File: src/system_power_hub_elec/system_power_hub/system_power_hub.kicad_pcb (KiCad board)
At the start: 6 copper layers, 65 x 65 mm, 127 parts, among them J1 XT90M, J101 SM02B-PASS, J2 XT60F, J3 SM02B-PASS, J4 XT60F, J6 IDC6, J8 XT60F, J9 XT60F, Q1 SSM3K333R, Q10 IRFH7440TRPBF, Q2 Q_Dual_NPN_NPN_E1B1C2E2B2C1, Q3 IRFH7440TRPBF, Q4 IRFH7440TRPBF, Q8 Q_Dual_NPN_NPN_E1B1C2E2B2C1, Q9 IRFH7440TRPBF, U102 TCAN1462V, U2 STM32G474RBT6, U220 MP2459GJ-Z-MS, U230 AP62200TWU, U4 24LC128, Y1 24MHz

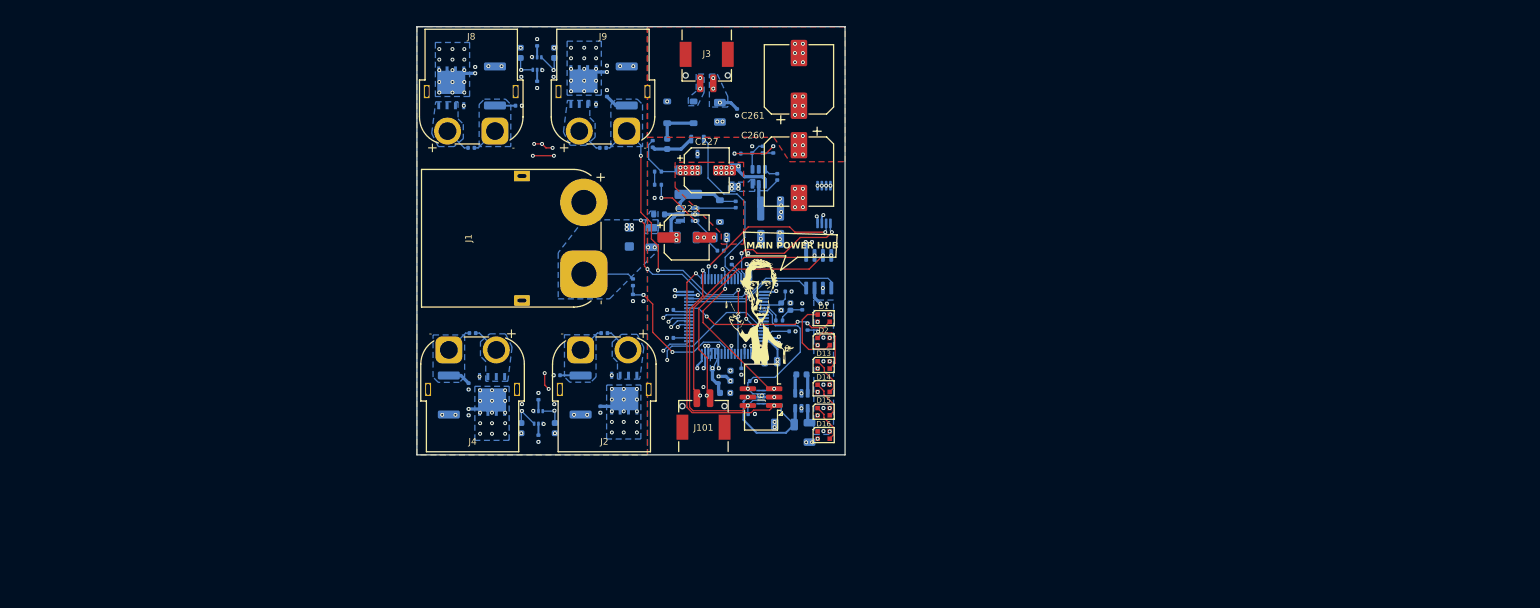
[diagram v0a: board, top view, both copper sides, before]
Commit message: Draft SPM PCB layout
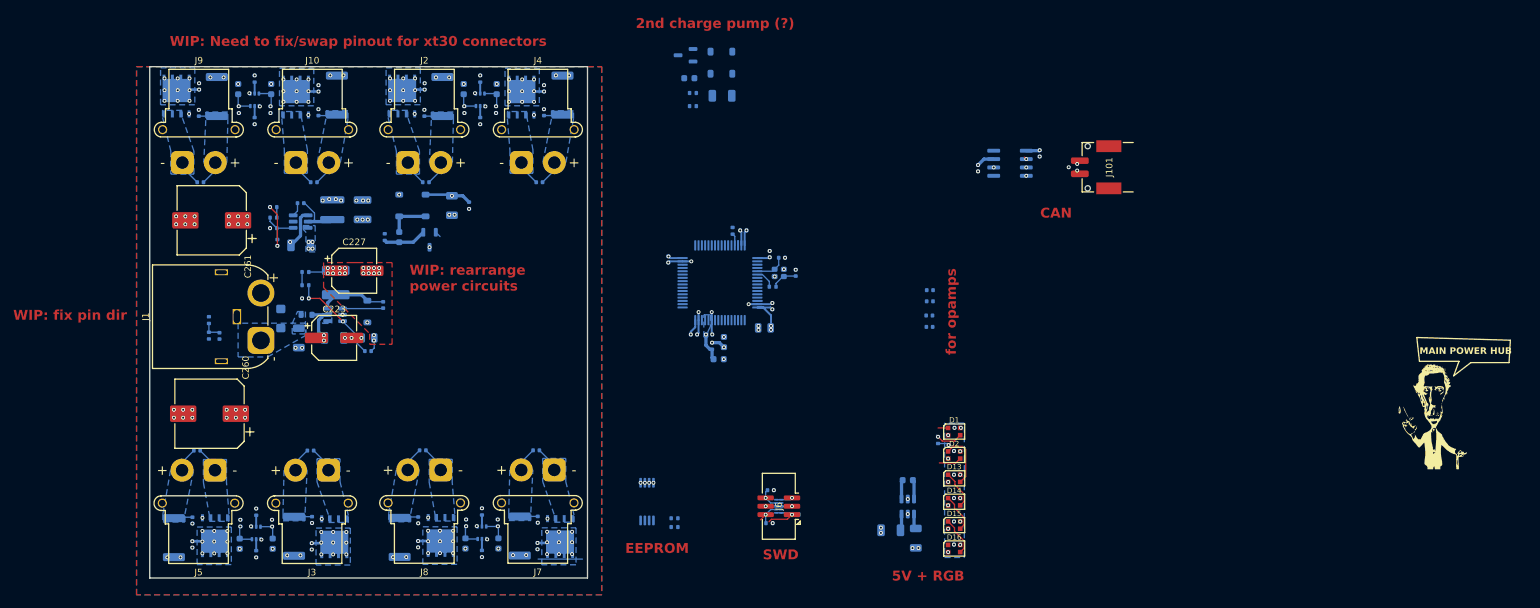
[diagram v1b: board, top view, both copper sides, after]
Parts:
- removed U2: STM32G474RBT6, Package_QFP:LQFP-64_10x10mm_P0.5mm
- added C32: 100n, Capacitor_SMD:C_0603_1608Metric, B.Cu at (141.4, 57.8)
- added C33: 1u, Capacitor_SMD:C_1206_3216Metric, B.Cu at (146.3, 60.5)
- added C34: 100n, Capacitor_SMD:C_0603_1608Metric, B.Cu at (78.1, 128.5)
- added C35: 100n, Capacitor_SMD:C_0603_1608Metric, B.Cu at (73.1, 128.5)
- added C38: 1n, Capacitor_SMD:C_0402_1005Metric, B.Cu at (83.8, 114.4)
- added C39: 1n, Capacitor_SMD:C_0402_1005Metric, B.Cu at (84.1, 124.9)
- added C40: 1n, Capacitor_SMD:C_0402_1005Metric, B.Cu at (66.6, 114.4)
- added C41: 1n, Capacitor_SMD:C_0402_1005Metric, B.Cu at (65.9, 125.0)
- added C42: 100n, Capacitor_SMD:C_0603_1608Metric, B.Cu at (112.4, 128.4)
- added C43: 100n, Capacitor_SMD:C_0603_1608Metric, B.Cu at (107.4, 128.5)
- added C44: 1n, Capacitor_SMD:C_0402_1005Metric, B.Cu at (118.1, 114.3)
- added C45: 1n, Capacitor_SMD:C_0402_1005Metric, B.Cu at (118.3, 124.8)
- added C46: 1n, Capacitor_SMD:C_0402_1005Metric, B.Cu at (100.9, 114.3)
- added C47: 1n, Capacitor_SMD:C_0402_1005Metric, B.Cu at (100.2, 124.9)
- added C48: 1n, Capacitor_SMD:C_0402_1005Metric, B.Cu at (118.3, 128.9)
- added C49: 1n, Capacitor_SMD:C_0402_1005Metric, B.Cu at (100.2, 128.6)
- added C50: 1n, Capacitor_SMD:C_0402_1005Metric, B.Cu at (84.0, 128.9)
- added C51: 1n, Capacitor_SMD:C_0402_1005Metric, B.Cu at (65.9, 128.6)
- added D4: SBR0560S1-7, Diode_SMD:D_SOD-123, B.Cu at (146.2, 53.8)
- added D5: SBR0560S1-7, Diode_SMD:D_SOD-123, B.Cu at (146.2, 57.1)
- added J5: XT30F, Connector_AMASS:AMASS_XT30PW-F_1x02_P2.50mm_Horizontal, F.Cu at (69.3, 117.3)
- added J7: XT30F, Connector_AMASS:AMASS_XT30PW-F_1x02_P2.50mm_Horizontal, F.Cu at (120.8, 117.3)
- added J8: XT30F, Connector_AMASS:AMASS_XT30PW-F_1x02_P2.50mm_Horizontal, F.Cu at (103.6, 117.3)
- added Q10: IRFH7440TRPBF, Bluesat:PQFN_5x6mm_E_SGD, B.Cu at (103.6, 127.6)
- added Q11: IRFH7440TRPBF, Bluesat:PQFN_5x6mm_E_SGD, B.Cu at (69.4, 127.6)
- added Q5: SSM3K333R, Package_TO_SOT_SMD:SOT-23-3, B.Cu at (140.8, 54.3)
- added Q6: Q_Dual_NPN_NPN_E1B1C2E2B2C1, Package_TO_SOT_SMD:SOT-363_SC-70-6, B.Cu at (75.6, 126.9)
- added Q7: IRFH7440TRPBF, Bluesat:PQFN_5x6mm_E_SGD, B.Cu at (87.5, 127.8)
- added Q8: Q_Dual_NPN_NPN_E1B1C2E2B2C1, Package_TO_SOT_SMD:SOT-363_SC-70-6, B.Cu at (109.9, 126.8)
- added Q9: IRFH7440TRPBF, Bluesat:PQFN_5x6mm_E_SGD, B.Cu at (121.7, 127.7)
- added R16: 10k, Resistor_SMD:R_0402_1005Metric, B.Cu at (109.9, 130.0)
- added R18: 100R, Resistor_SMD:R_0402_1005Metric, B.Cu at (141.9, 60.1)
- added R20: 470k, Resistor_SMD:R_0402_1005Metric, B.Cu at (141.9, 62.1)
- added R21: 10k, Resistor_SMD:R_0402_1005Metric, B.Cu at (109.9, 123.6)
- added R22: 470k, Resistor_SMD:R_0402_1005Metric, B.Cu at (112.3, 125.3)
- added R23: 470k, Resistor_SMD:R_0402_1005Metric, B.Cu at (107.5, 125.3)
- added R24: 10k, Resistor_SMD:R_0402_1005Metric, B.Cu at (75.6, 130.1)
- added R25: 10k, Resistor_SMD:R_0402_1005Metric, B.Cu at (75.6, 123.7)
- added R26: 1m, Resistor_SMD:R_2512_6332Metric, B.Cu at (115.6, 127.3)
- added R27: 1m, Resistor_SMD:R_2512_6332Metric, B.Cu at (97.4, 127.5)
- added R28: 470k, Resistor_SMD:R_0402_1005Metric, B.Cu at (78.0, 125.4)
- added R29: 470k, Resistor_SMD:R_0402_1005Metric, B.Cu at (73.2, 125.4)
- added R30: 1m, Resistor_SMD:R_2512_6332Metric, B.Cu at (81.3, 127.4)
- added R31: 1m, Resistor_SMD:R_2512_6332Metric, B.Cu at (63.1, 127.6)
- added U1: STM32G474RBT6, Package_QFP:LQFP-64_10x10mm_P0.5mm, B.Cu at (146.0, 88.9)
- J1: value XT90M -> XT60M; footprint Connector_AMASS:AMASS_XT90PW-M_1x02_P10.90mm_Horizontal -> Connector_AMASS:AMASS_XT60IPW-M_1x03_P7.20mm_Horizontal
- J10: renamed from J9; value XT60F -> XT30F; footprint Connector_AMASS:AMASS_XT60PW-F_1x02_P7.20mm_Horizontal -> Connector_AMASS:AMASS_XT30PW-F_1x02_P2.50mm_Horizontal
- J2, J4: value XT60F -> XT30F; footprint Connector_AMASS:AMASS_XT60PW-F_1x02_P7.20mm_Horizontal -> Connector_AMASS:AMASS_XT30PW-F_1x02_P2.50mm_Horizontal
- J3: value SM02B-PASS -> XT30F; footprint Bluesat:SM02B-PASS -> Connector_AMASS:AMASS_XT30PW-F_1x02_P2.50mm_Horizontal
- J9: renamed from J8; value XT60F -> XT30F; footprint Connector_AMASS:AMASS_XT60PW-F_1x02_P7.20mm_Horizontal -> Connector_AMASS:AMASS_XT30PW-F_1x02_P2.50mm_Horizontal
- moved G*** 103.4 mm to (254.4, 108.5)
- moved C260 96.7 mm to (68.5, 108.8), turned to 180 degrees
- moved C261 91.7 mm to (68.8, 79.4), turned to 180 degrees
- moved J3 88.5 mm to (86.6, 117.3), turned to 180 degrees
- moved J101 78.9 mm to (209.2, 71.3), turned to -90 degrees
- moved R230 76.4 mm to (78.2, 77.4), turned to 0 degrees
- moved R231 75.0 mm to (78.2, 79.0), turned to 180 degrees
- moved R232 73.7 mm to (78.2, 80.6), turned to 180 degrees
- moved C231 72.5 mm to (82.4, 76.8), turned to 0 degrees
- moved C232 71.2 mm to (78.8, 82.8), turned to -90 degrees
- moved U230 69.9 mm to (82.4, 79.6), turned to 180 degrees
- moved C230 66.8 mm to (82.4, 83.2), turned to 0 degrees
- moved L230 66.5 mm to (87.2, 77.8), turned to 90 degrees
- moved D101 65.6 mm to (199.6, 71.3), turned to 180 degrees
- moved C12 64.6 mm to (70.0, 96.9)
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- renumbered C to C1, C to C250, C42 to C52, C43 to C53, C44 to C54, C45 to C55, C46 to C56, C47 to C57, C48 to C58, C49 to C59, Q4 to Q12, Q8 to Q13, Q9 to Q15, Q10 to Q16, Q3 to Q4, R16 to R32, R21 to R33, R22 to R34, R23 to R35, R26 to R36, R27 to R37, U to U240
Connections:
- C15 pad 1: GND -> Net-(U1A-PA2-opamp_vout_0)
- C16 pad 1: GND -> Net-(U1A-PA8-opamp_vout_1)
- C17 pad 1: GND -> Net-(U1A-PA6-opamp_vout_2)
- C18 pad 1: GND -> Net-(U1A-PB11-opamp_vout_3)
- D12 pad 1: Net-(D12-K) -> Vdrive
- J1 pad 1: VBUS -> GND
- J1 pad 2: GND -> VBUS
- J3 pad 1: Vdrive -> /Analog Stuff/vsense_p4
- J3 pad 2: Net-(D12-K) -> Net-(J3-Pin_2)
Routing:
- net /Analog Stuff/vsense_p3: track 87.1 -> 10.5 mm, vias 1 -> 0
- net Vdrive: track 138.0 -> 78.8 mm, vias 12 -> 9
- net /Analog Stuff/vsense_p0: track 68.7 -> 10.4 mm, vias 6 -> 0
- net /Analog Stuff/~{chan0}: track 57.8 -> 0.00 mm, vias 2 -> 1
- net /Analog Stuff/~{chan1}: track 54.5 -> 0.00 mm, vias 2 -> 1
- net /Analog Stuff/vsense_p1: track 54.7 -> 10.5 mm, vias 4 -> 0
- net /Analog Stuff/~{chan2}: track 39.1 -> 0.00 mm, vias 2 -> 1
- net /CANH: track 35.9 -> 0.11 mm
- net /CANL: track 35.4 -> 0.42 mm
- net /dbg.swdio: track 38.9 -> 6.46 mm, vias 2 -> 1
- net /dbg.swclk: track 36.5 -> 5.13 mm, vias 2 -> 1
- net /Analog Stuff/~{chan3}: track 28.4 -> 0.00 mm, vias 2 -> 1
- net /Analog Stuff/clk_in: track 27.5 -> 0.92 mm
- net Net-(U102-TXD): track 24.1 -> 0.07 mm
- net /dbg.swo: track 27.1 -> 3.26 mm, vias 3 -> 1
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- added copper zone on B.Cu, net /Analog Stuff/vsense_p4
- added copper zone on B.Cu, net /Analog Stuff/vsense_p5
- added copper zone on B.Cu, net /Analog Stuff/vsense_p6
- added copper zone on B.Cu, net /Analog Stuff/vsense_p7
- added copper zone on B.Cu, net Net-(J3-Pin_2)
- added copper zone on B.Cu, net Net-(J7-Pin_2)
- added copper zone on B.Cu, net Net-(J8-Pin_2)
- removed copper zone on B.Cu, net Net-(D12-K)
- removed copper zone on B.Cu, net Net-(J2-Pin_2)
- removed copper zone on In3.Cu, net VDD
- removed copper zone on B.Cu, net Vdrive
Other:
- board size 65 x 65 mm -> 66.5 x 77.6 mm
- board text added: "2nd charge pump (?)"
- board text added: "5V + RGB"
- board text added: "CAN"
- board text added: "EEPROM"
- board text added: "SWD"
- board text added: "WIP: Need to fix/swap pinout for xt30 connectors"
- board text added: "WIP: fix pin dir"
- board text added: "WIP: rearrange power circuits"
- board text added: "for opamps"
